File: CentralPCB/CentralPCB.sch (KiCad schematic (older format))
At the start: 56 parts, among them J1 POWER HEADER, J2 SPI Header, J3 Conn_02x16_Odd_Even, J4 Conn_Coaxial, J5 Conn_02x10_Odd_Even, J6 Conn_01x05, U1 AD8531, U2 Teensy4.1, U3 BA7810CP-E2

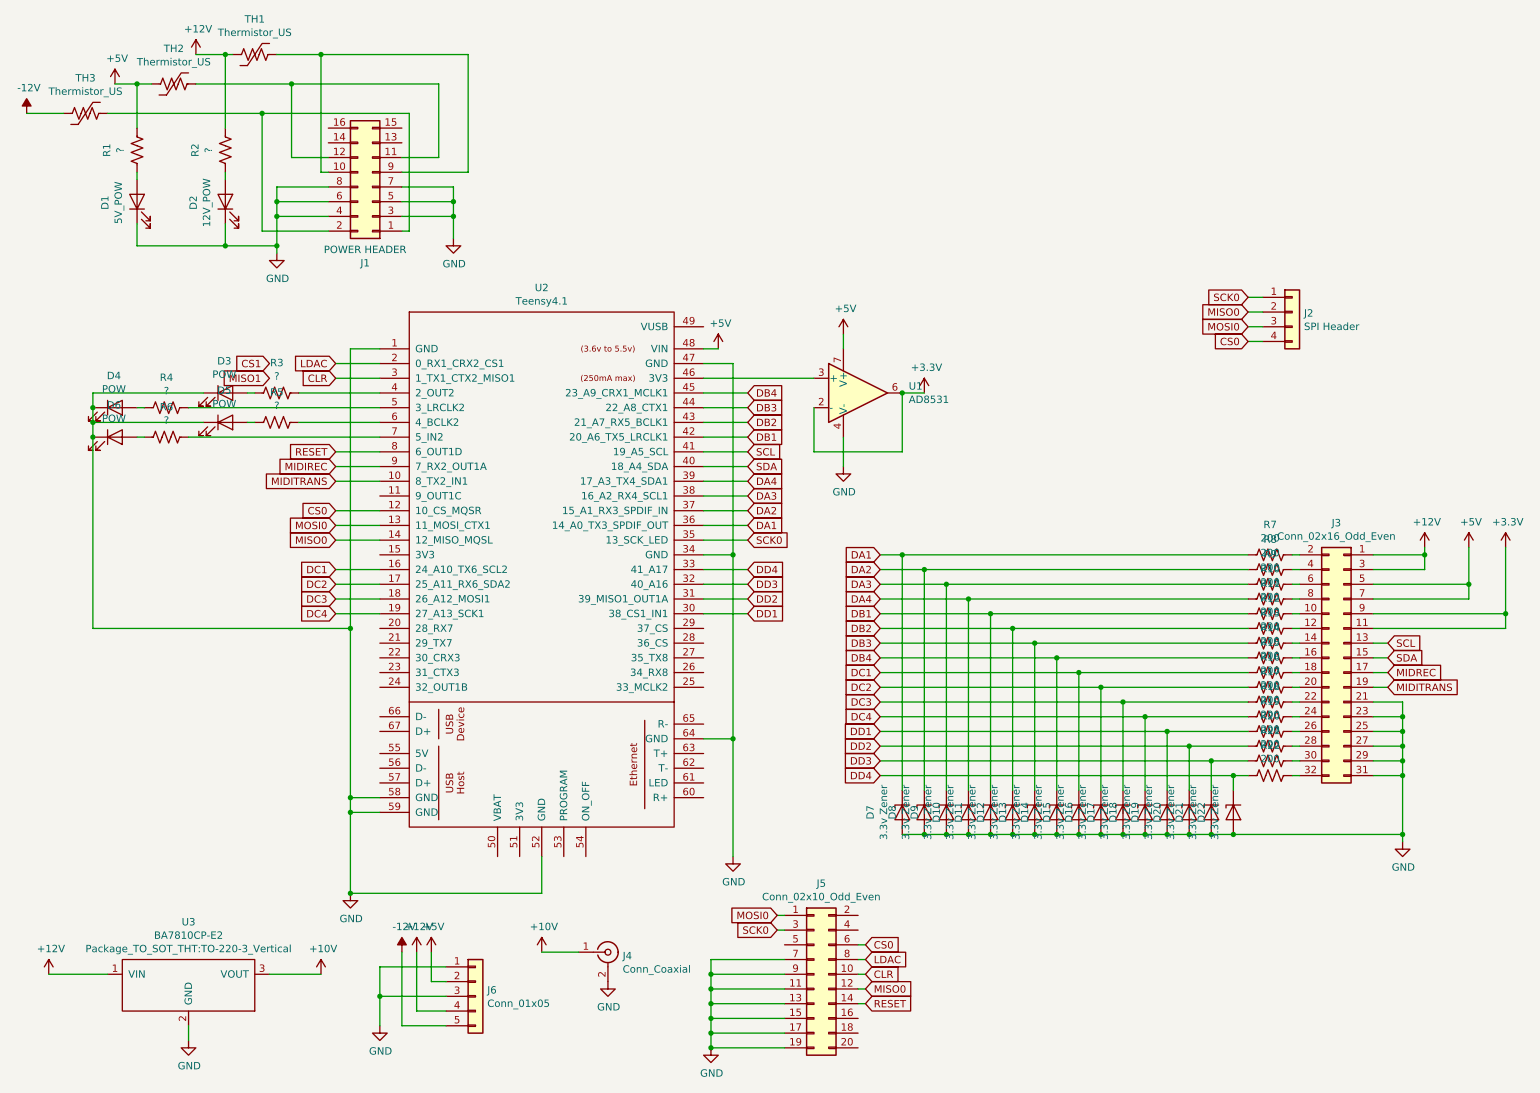
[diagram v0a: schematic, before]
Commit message: Pin updates
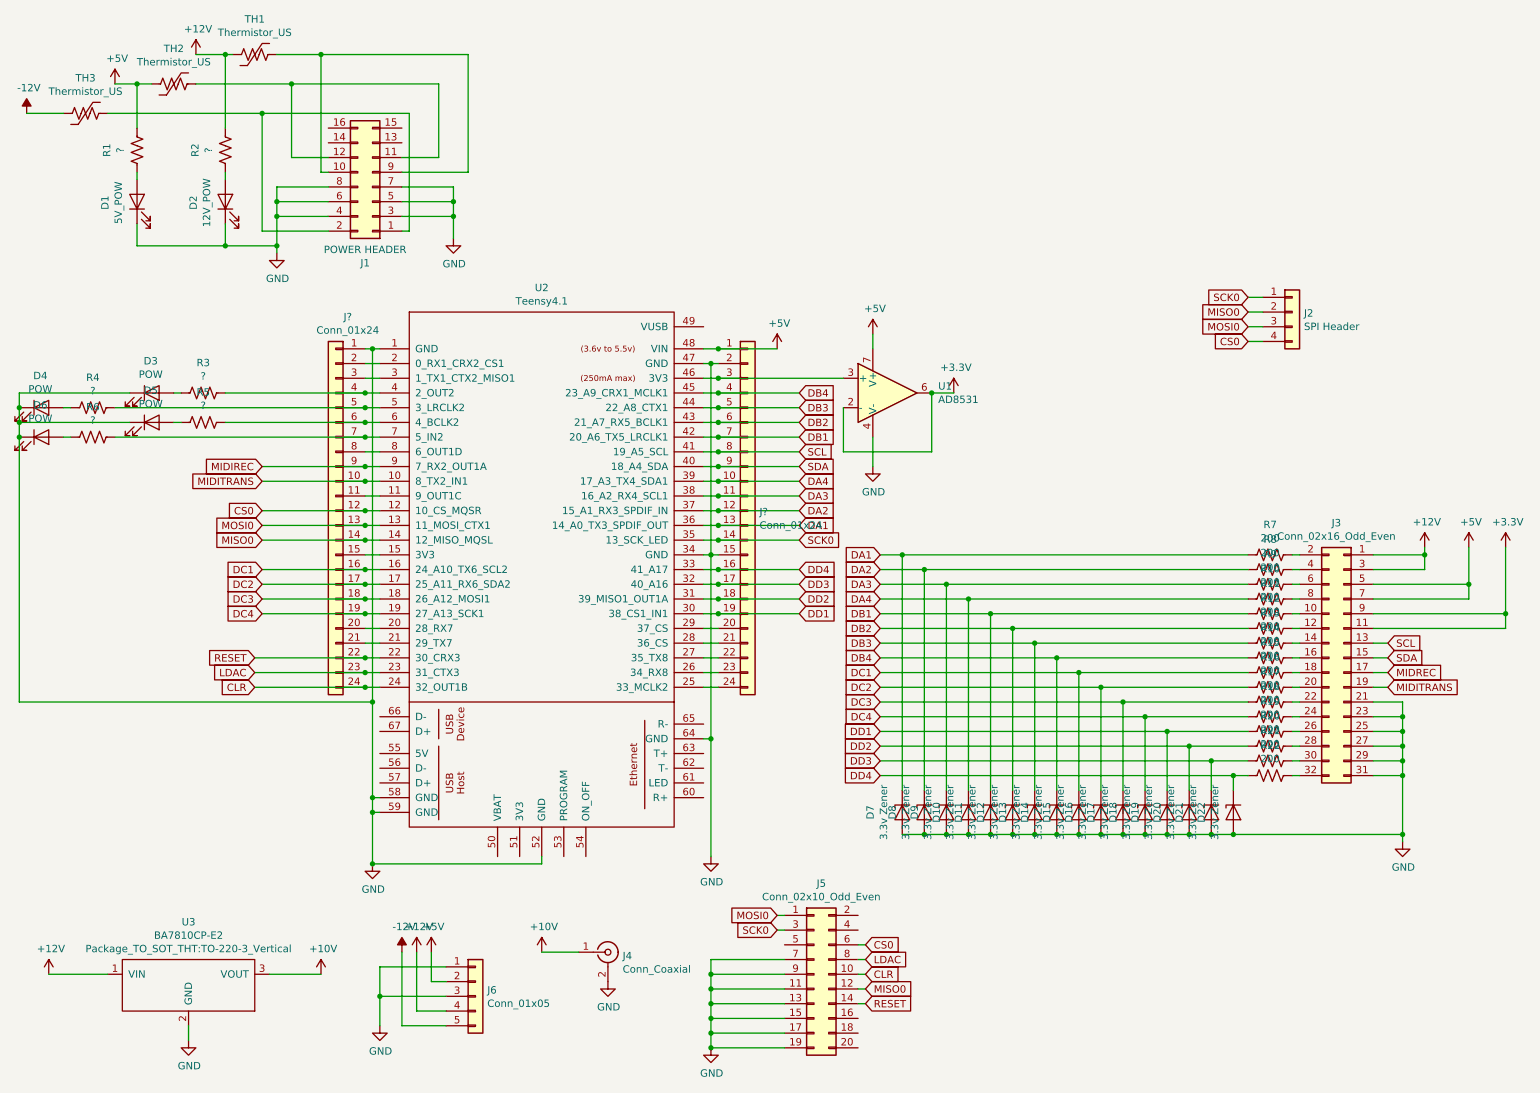
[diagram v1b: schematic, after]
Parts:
- added J? (x2): Conn_01x24, Connector_PinSocket_2.54mm:PinSocket_1x23_P2.54mm_Vertical, symbol Connector_Generic:Conn_01x24
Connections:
- net +5V: now also J?.1 (Pin_1)
- net CLR: now also U2.24 (32_OUT1B), J?.24 (Pin_24); no longer U2.3 (1_TX1_CTX2_MISO1)
- net CS0: now also J?.12 (Pin_12)
- net DA1: now also J?.13 (Pin_13)
- net DA2: now also J?.12 (Pin_12)
- net DA3: now also J?.11 (Pin_11)
- net DA4: now also J?.10 (Pin_10)
- net DB1: now also J?.7 (Pin_7)
- net DB2: now also J?.6 (Pin_6)
- net DB3: now also J?.5 (Pin_5)
- net DB4: now also J?.4 (Pin_4)
- net DC1: now also J?.16 (Pin_16)
- net DC2: now also J?.17 (Pin_17)
- net DC3: now also J?.18 (Pin_18)
- net DC4: now also J?.19 (Pin_19)
- net DD1: now also J?.19 (Pin_19)
- net DD2: now also J?.18 (Pin_18)
- net DD3: now also J?.17 (Pin_17)
- net DD4: now also J?.16 (Pin_16)
- net GND: now also J?.1 (Pin_1), J?.15 (Pin_15), J?.2 (Pin_2)
- net LDAC: now also U2.23 (31_CTX3), J?.23 (Pin_23); no longer U2.2 (0_RX1_CRX2_CS1)
- net MIDIREC: now also J?.9 (Pin_9)
- net MIDITRANS: now also J?.10 (Pin_10)
- net MISO0: now also J?.14 (Pin_14)
- net MOSI0: now also J?.13 (Pin_13)
- net RESET: now also U2.22 (30_CRX3), J?.22 (Pin_22); no longer U2.8 (6_OUT1D)
- net SCK0: now also J?.14 (Pin_14)
- net SCL: now also J?.8 (Pin_8)
- net SDA: now also J?.9 (Pin_9)
- net at R3.1, U2.4 (2_OUT2): now also J?.4 (Pin_4)
- net at R4.1, U2.5 (3_LRCLK2): now also J?.5 (Pin_5)
- net at R5.1, U2.6 (4_BCLK2): now also J?.6 (Pin_6)
- net at R6.1, U2.7 (5_IN2): now also J?.7 (Pin_7)
- net at U2.11 (9_OUT1C): now also J?.11 (Pin_11)
- net at U2.15 (3V3): now also J?.15 (Pin_15)
- net at U2.20 (28_RX7): now also J?.20 (Pin_20)
- net at U2.21 (29_TX7): now also J?.21 (Pin_21)
- net at U2.25 (33_MCLK2): now also J?.24 (Pin_24)
- net at U2.26 (34_RX8): now also J?.23 (Pin_23)
- net at U2.27 (35_TX8): now also J?.22 (Pin_22)
- net at U2.28 (36_CS): now also J?.21 (Pin_21)
- net at U2.29 (37_CS): now also J?.20 (Pin_20)
- net at U1.3 (+), U2.46 (3V3): now also J?.3 (Pin_3)
- new net: J?.2 (Pin_2), U2.2 (0_RX1_CRX2_CS1)
- new net: J?.3 (Pin_3), U2.3 (1_TX1_CTX2_MISO1)
- new net: J?.8 (Pin_8), U2.8 (6_OUT1D)
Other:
- moved on the sheet: D3, D4, D5, D6, R3, R4, R5, R6, U1
